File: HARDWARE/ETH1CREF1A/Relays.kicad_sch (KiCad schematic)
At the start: 37 parts, among them J901 Conn_02x06_Odd_Even, K901 9012, K902 9012, K903 9012, K904 9012, K905 9012, K906 9012, K907 9012, K908 9012, K909 9012, K910 9012, K911 9012, K912 9012, K913 9012, K914 9012, K915 9012, K916 9012, K917 9012, K918 9012

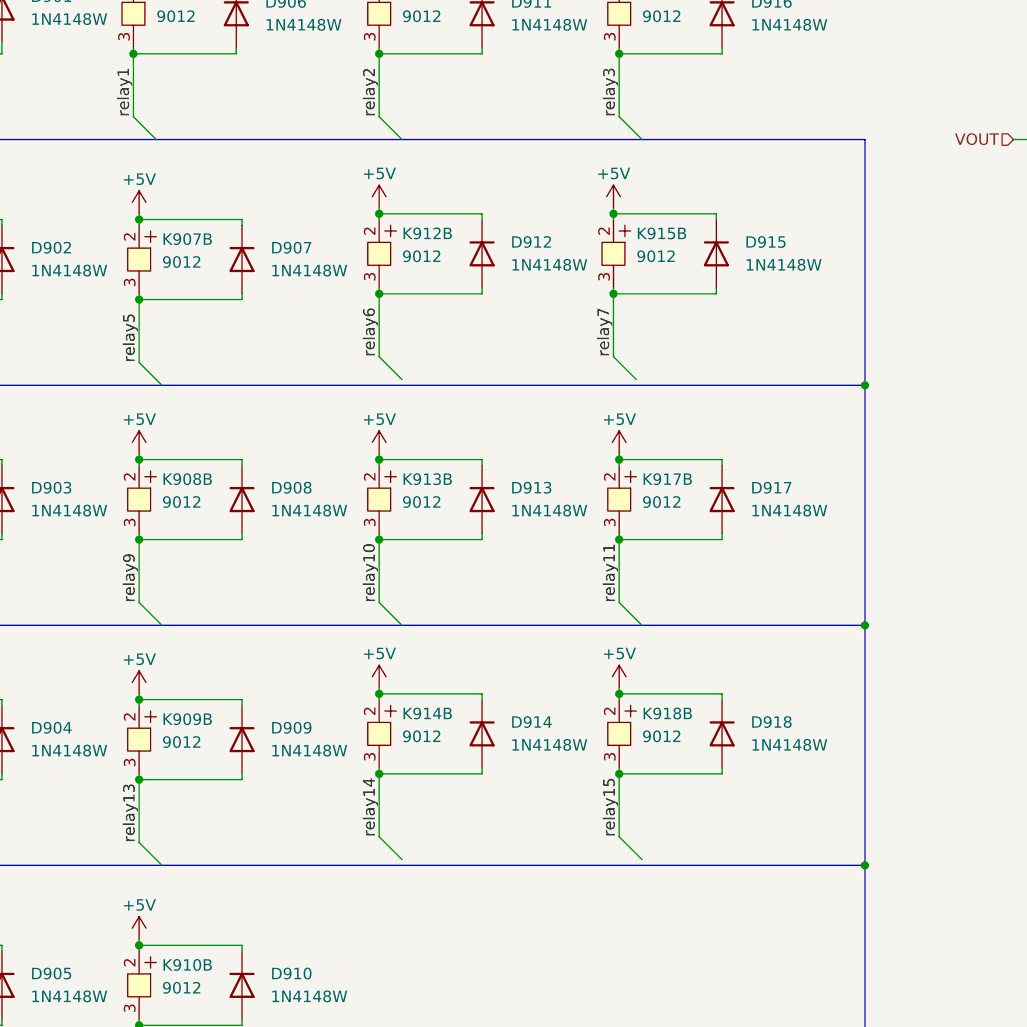
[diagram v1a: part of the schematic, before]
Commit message: Hardware
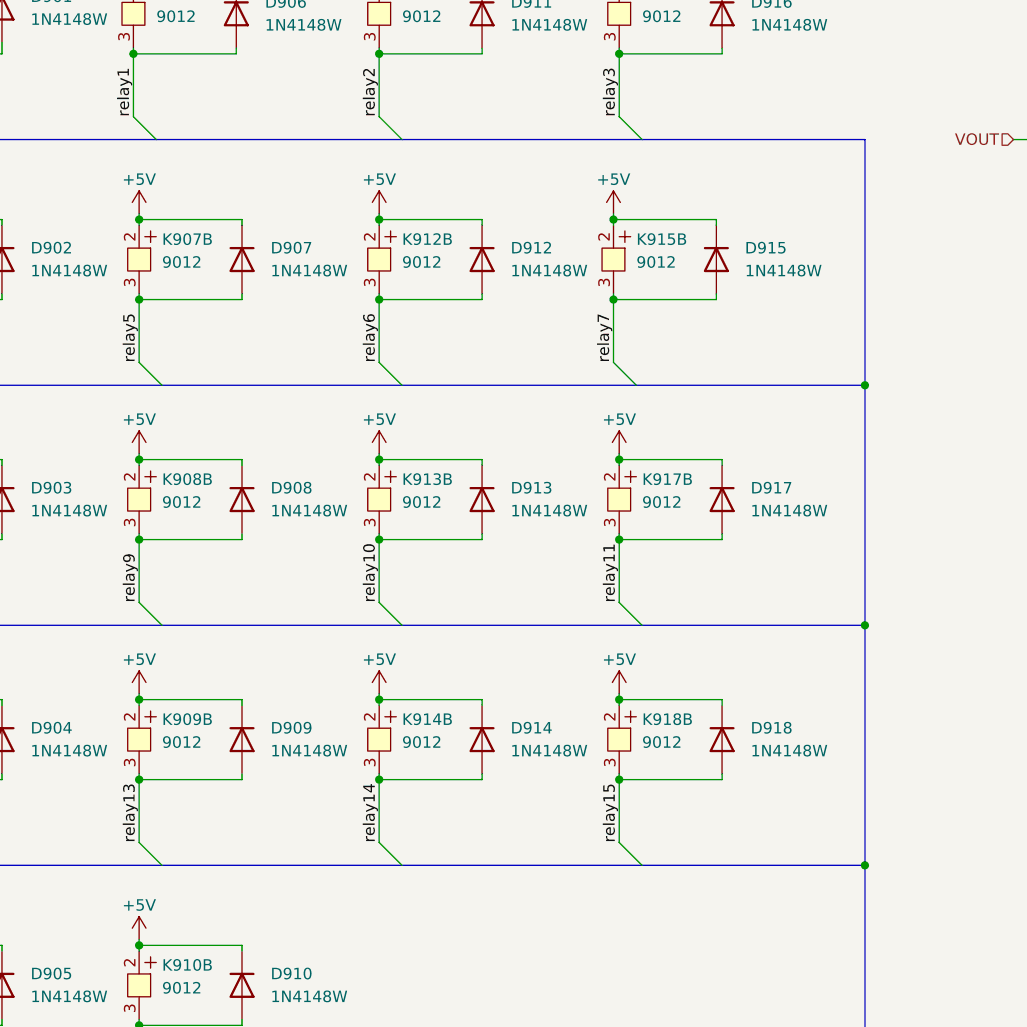
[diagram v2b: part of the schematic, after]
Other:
- moved on the sheet: D912, D914, D915, D918, K912B, K914B, K915B, K918B
